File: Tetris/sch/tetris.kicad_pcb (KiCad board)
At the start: 2 copper layers, 33 x 91.4 mm, 76 parts, among them J1 SWD, Q1 HL4953A, Q2 HL4953A, Q3 HL4953A, Q4 HL4953A, SW1 Boot, SW3 TSX101G100-250, SW4 Reset, U1 CH32V203C8T6, U10 ZX-QC66-6.5CJ, U11 MCP6001T-I/OT-TUDI, U2 STP16CP05TTR, U3 74HCT595D, U4 TLV70433DBVR, U5 SZ421288N/64, U6 SZ421288N/64, U7 LM1085-ADJ, U8 ZX-QC66-6.5CJ, U9 ZX-QC66-6.5CJ

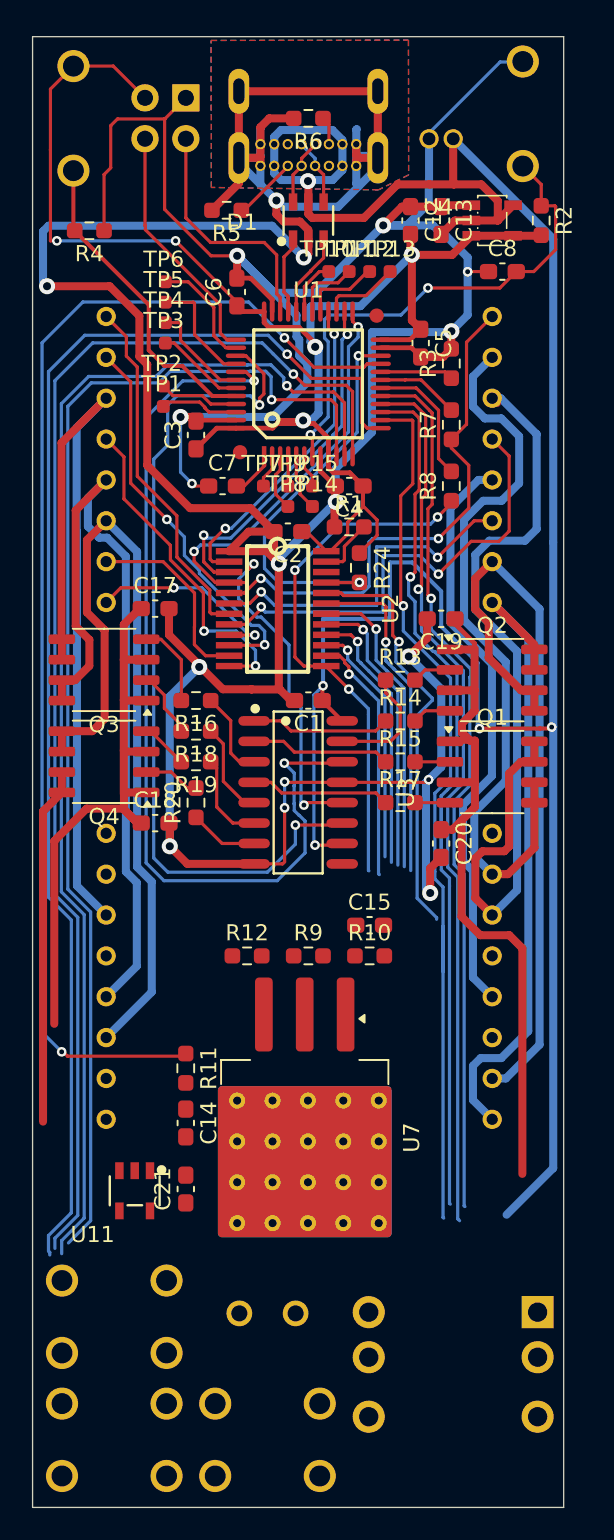
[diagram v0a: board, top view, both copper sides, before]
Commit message: PCB is ready
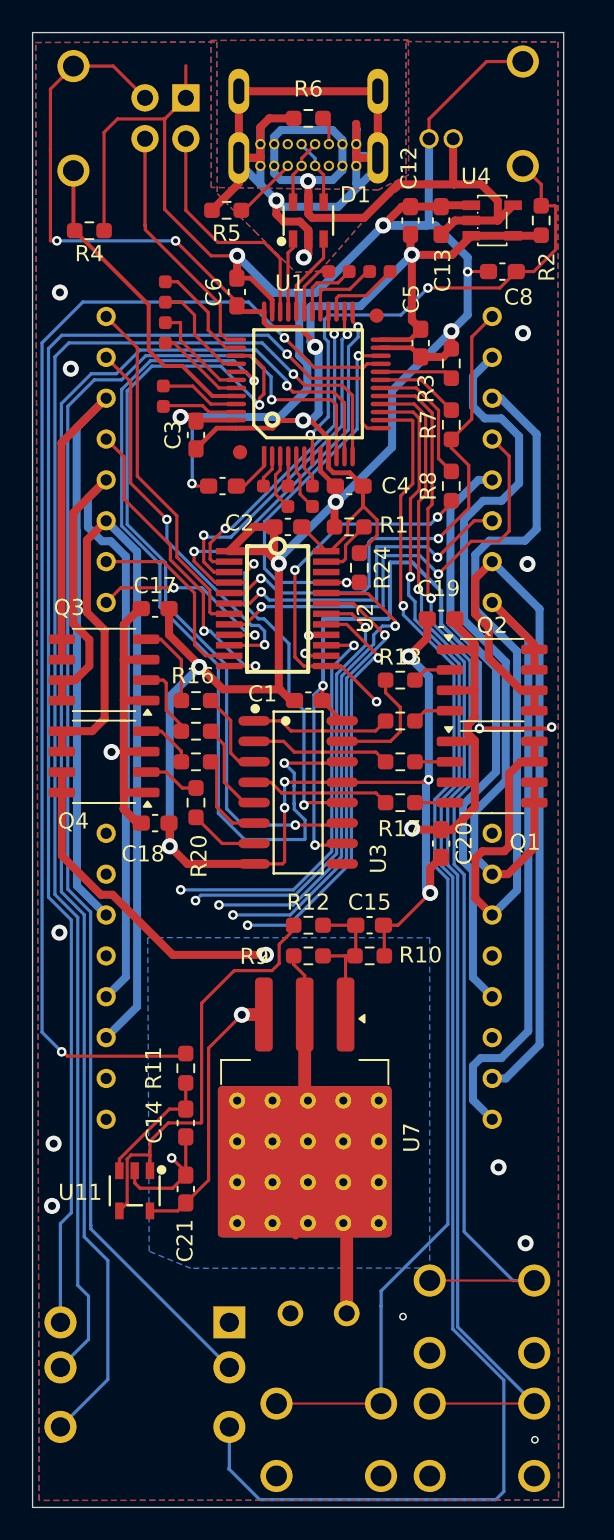
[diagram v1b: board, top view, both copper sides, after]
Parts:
- moved U10 22.9 mm to (127.0, 119.6)
- moved U8 22.9 mm to (127.0, 127.2)
- moved SW3 19.2 mm to (106.0, 123.2)
- moved R12 4.26 mm to (116.2, 95.2)
- moved U9 3.81 mm to (117.5, 127.2)
- moved C11 3.17 mm to (116.8, 119.4)
- moved C2 0.30 mm to (114.9, 70.5)
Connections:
- U1 pad 11: /Btns/B2 -> /Btns/B5
- U1 pad 12: /Btns/B3 -> /Btns/B4
- U1 pad 13: /Btns/B4 -> /Btns/B3
- U1 pad 14: /Btns/B5 -> /Btns/B7
- U1 pad 15: /Btns/B6 -> /Btns/B2
- U1 pad 16: /Btns/B7 -> /Btns/B6
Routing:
- net /LED/LED-Pwr: track 84.4 -> 125.5 mm, vias 0 -> 2
- net /Btns/B5: track 56.7 -> 89.9 mm
- net Net-(U11--IN): track 0.00 -> 26.5 mm
- net +5V: track 153.3 -> 179.5 mm, vias 5 -> 6
- net Net-(U2-~{OUT12}): track 18.0 -> 41.5 mm, vias 1 -> 2
- net Net-(U2-~{OUT14}): track 20.9 -> 41.3 mm, vias 1 -> 2
- net /Btns/B7: track 55.3 -> 73.8 mm
- net /Btns/B6: track 57.4 -> 75.1 mm
- net /Btns/B2: track 77.1 -> 93.6 mm
- net Net-(U2-~{OUT10}): track 15.3 -> 31.6 mm, vias 1 -> 2
- net Net-(U2-~{OUT9}): track 15.6 -> 31.9 mm
- net Net-(U2-~{OUT13}): track 19.0 -> 33.8 mm, vias 1 -> 2
- net Net-(U5-COL1): track 58.5 -> 72.1 mm, vias 0 -> 1
- net /Btns/B8: track 55.0 -> 68.5 mm
- net Net-(U2-~{OUT15}): track 26.2 -> 38.7 mm, vias 1 -> 2
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- added copper zone on In1.Cu, net +3V3
- added copper zone on B.Cu, net /LED/LED-Pwr
- added copper zone on In1.Cu, net GND
- added copper zone on In2.Cu, net GND
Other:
- board size 33 x 91.4 mm -> 33 x 91.7 mm
- copper layers 2 -> 4
- rule pad_to_mask_clearance: 0.05 -> 0
- board text added: "Boot"
- board text added: "Reset"
